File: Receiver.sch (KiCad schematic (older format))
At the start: 29 parts, among them J1 +12V, J2 -12V, J3 GND, J4 OUTPUT, U1 TL074 (ggf. durch TLV4172IPWR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

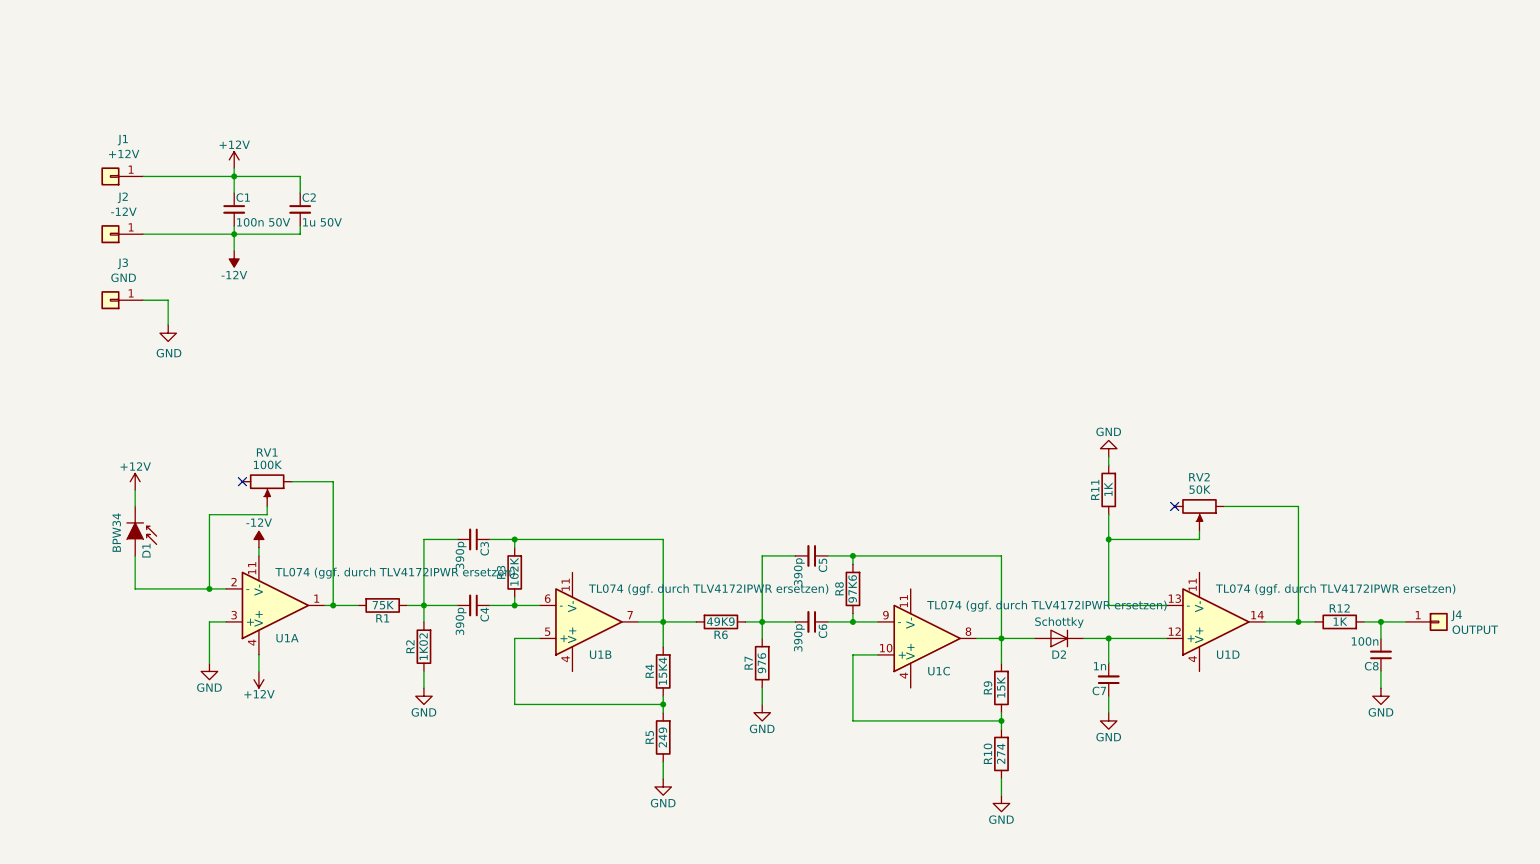
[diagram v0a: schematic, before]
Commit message: Update schematic and pcb
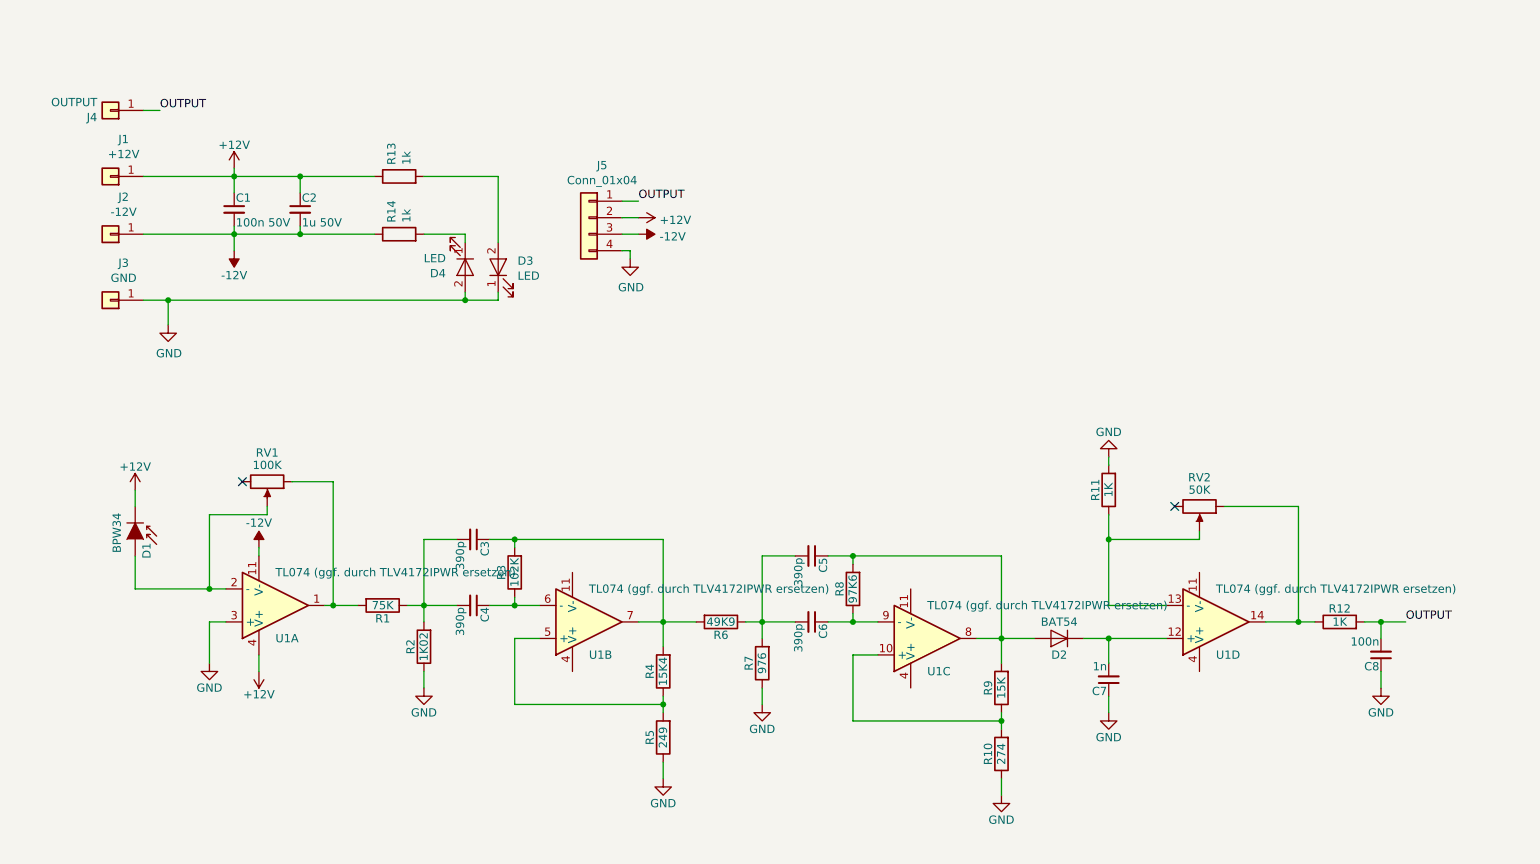
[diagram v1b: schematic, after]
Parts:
- added D3, D4: LED, LEDs:LED_0603, symbol device:LED
- added J5: Conn_01x04, Pin_Headers:Pin_Header_Straight_1x04_Pitch2.54mm, symbol Connector:Conn_01x04
- added R13, R14: 1k, Resistors_SMD:R_0603, symbol device:R
- D2: value Schottky -> BAT54; footprint Diodes_SMD:D_SOD-123 -> Diodes_SMD:D_SOT-23_ANK
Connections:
- net +12V: now also J5.2 (Pin_2), R13.1
- net -12V: now also J5.3 (Pin_3), R14.1
- net GND: now also D3.1 (K), D4.2 (A), J5.4 (Pin_4)
- net OUTPUT: now reaches C8.2, J4.1 (Pin_1), R12.2
- net OUTPUT: now also J5.1 (Pin_1)
- new net: D3.2 (A), R13.2
- new net: D4.1 (K), R14.2
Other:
- moved on the sheet: J4
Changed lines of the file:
@@
 P 7700 4300
 F 0 "D2" H 7700 4400 50  0000 C CNN
-F 1 "Schottky " H 7700 4200 50  0000 C CNN
-F 2 "Diodes_SMD:D_SOD-123" H 7700 4300 50  0001 C CNN
+F 1 "BAT54" H 7700 4200 50  0000 C CNN
+F 2 "Diodes_SMD:D_SOT-23_ANK" H 7700 4300 50  0001 C CNN
 F 3 "" H 7700 4300 50  0001 C CNN
 	1    7700 4300
@@
 L Connector:Conn_01x01 J4
 U 1 1 5B03236E
-P 10000 4200
-F 0 "J4" H 10080 4242 50  0000 L CNN
-F 1 "OUTPUT" H 10080 4151 50  0000 L CNN
-F 2 "optoreceiver:Hirschmann_MST201" H 10000 4200 50  0001 C CNN
-F 3 "~" H 10000 4200 50  0001 C CNN
-	1    10000 4200
-	1    0    0    -1
+P 1950 1100
+F 0 "J4" H 2030 1142 50  0000 L CNN
+F 1 "OUTPUT" H 2030 1051 50  0000 L CNN
+F 2 "optoreceiver:Hirschmann_MST201" H 1950 1100 50  0001 C CNN
+F 3 "~" H 1950 1100 50  0001 C CNN
+	1    1950 1100
+	-1   0    0    1
 $EndComp
 Wire Wire Line
@@
 Wire Wire Line
 	2300 2250 2300 2400
+$Comp
+L device:LED D3
+U 1 1 5B14466C
+P 4300 2050
+F 0 "D3" V 4338 1933 50  0000 R CNN
+F 1 "LED" V 4247 1933 50  0000 R CNN
+F 2 "LEDs:LED_0603" H 4300 2050 50  0001 C CNN
+F 3 "~" H 4300 2050 50  0001 C CNN
+	1    4300 2050
+	0    -1   -1   0
+$EndComp
+Wire Wire Line
+	4300 2200 4300 2250
+$Comp
+L device:R R13
+U 1 1 5B14B3A1
+P 3700 1500
+F 0 "R13" H 3770 1546 50  0000 L CNN
+F 1 "1k" H 3770 1455 50  0000 L CNN
+F 2 "Resistors_SMD:R_0603" V 3630 1500 50  0001 C CNN
+F 3 "" H 3700 1500 50  0001 C CNN
+	1    3700 1500
+	0    -1   -1   0
+$EndComp
+$Comp
+L Connector:Conn_01x04 J5
+U 1 1 5B150E6D
+P 4850 1750
+F 0 "J5" H 4770 2067 50  0000 C CNN
+F 1 "Conn_01x04" H 4770 1976 50  0000 C CNN
+F 2 "Pin_Headers:Pin_Header_Straight_1x04_Pitch2.54mm" H 4850 1750 50  0001 C CNN
+F 3 "~" H 4850 1750 50  0001 C CNN
+	1    4850 1750
+	-1   0    0    -1
+$EndComp
+Text Label 2250 1100 0    50   ~ 0
+OUTPUT
+Wire Wire Line
+	2250 1100 2150 1100
+Text Label 9800 4200 0    50   ~ 0
+OUTPUT
+$Comp
+L power:GND #PWR0101
+U 1 1 5B156865
+P 5100 2000
+F 0 "#PWR0101" H 5100 1750 50  0001 C CNN
+F 1 "GND" H 5105 1827 50  0000 C CNN
+F 2 "" H 5100 2000 50  0001 C CNN
+F 3 "" H 5100 2000 50  0001 C CNN
+	1    5100 2000
+	1    0    0    -1
+$EndComp
+Wire Wire Line
+	5050 1950 5100 1950
+Wire Wire Line
+	5100 1950 5100 2000
+$Comp
+L power:+12V #PWR0102
+U 1 1 5B15914A
+P 5150 1750
+F 0 "#PWR0102" H 5150 1600 50  0001 C CNN
+F 1 "+12V" V 5165 1878 50  0000 L CNN
+F 2 "" H 5150 1750 50  0001 C CNN
+F 3 "" H 5150 1750 50  0001 C CNN
+	1    5150 1750
+	0    1    1    0
+$EndComp
+$Comp
+L power:-12V #PWR15
+U 1 1 5B15948E
+P 5150 1850
+F 0 "#PWR15" H 5150 1950 50  0001 C CNN
+F 1 "-12V" V 5165 1978 50  0000 L CNN
+F 2 "" H 5150 1850 50  0001 C CNN
+F 3 "" H 5150 1850 50  0001 C CNN
+	1    5150 1850
+	0    1    1    0
+$EndComp
+Wire Wire Line
+	5150 1850 5050 1850
+Wire Wire Line
+	5150 1750 5050 1750
+Text Label 5150 1650 0    50   ~ 0
+OUTPUT
+Wire Wire Line
+	5150 1650 5050 1650
+Wire Wire Line
+	3100 1500 3550 1500
+Connection ~ 3100 1500
+Wire Wire Line
+	2300 2250 4100 2250
+Connection ~ 2300 2250
+$Comp
+L device:R R14
+U 1 1 5B17749B
+P 3700 1850
+F 0 "R14" H 3770 1896 50  0000 L CNN
+F 1 "1k" H 3770 1805 50  0000 L CNN
+F 2 "Resistors_SMD:R_0603" V 3630 1850 50  0001 C CNN
+F 3 "" H 3700 1850 50  0001 C CNN
+	1    3700 1850
+	0    -1   -1   0
+$EndComp
+Wire Wire Line
+	3550 1850 3100 1850
+Connection ~ 3100 1850
+$Comp
+L device:LED D4
+U 1 1 5B182712
+P 4100 2050
+F 0 "D4" V 4138 1933 50  0000 R CNN
+F 1 "LED" V 4047 1933 50  0000 R CNN
+F 2 "LEDs:LED_0603" H 4100 2050 50  0001 C CNN
+F 3 "~" H 4100 2050 50  0001 C CNN
+	1    4100 2050
+	0    1    1    0
+$EndComp
+Wire Wire Line
+	4100 2200 4100 2250
+Connection ~ 4100 2250
+Wire Wire Line
+	4100 2250 4300 2250
+Wire Wire Line
+	3850 1850 4100 1850
+Wire Wire Line
+	4100 1850 4100 1900
+Wire Wire Line
+	3850 1500 4300 1500
+Wire Wire Line
+	4300 1500 4300 1900
 $EndSCHEMATC

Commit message: Add files via upload
- Platzierung und Silkscreen angepasst
- 3D Modelle ergänzt
- aktuelle Renderbilder erzeugt
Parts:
- C1, C2, C3, C4, C5, C6, C7, C8: symbol device:C_Small -> Device:C_Small
- D2: symbol device:D -> Device:D
- D3, D4: symbol device:LED -> Device:LED
- J1, J2, J3, J4: symbol Connector:Conn_01x01 -> Connector:Conn_01x01_Female
- J5: symbol Connector:Conn_01x04 -> Connector:Conn_01x04_Female
- R1, R10, R11, R12, R13, R14, R2, R3, R4, R5, R6, R7, R8, R9: symbol device:R -> Device:R
- RV1, RV2: footprint SparkFun-Electromechanical:TRIM_POT -> User-Submitted:BOURNS-3362P_pot
- U1: footprint Package_SO:TSSOP-14_4.4x5mm_P0.65mm -> Package_SO:SOIC-14_3.9x8.7mm_P1.27mm
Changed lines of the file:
@@
 F 0 "U1" H 2950 4300 50  0000 L CNN
 F 1 "TL074 (ggf. durch TLV4172IPWR ersetzen)" H 2950 3900 50  0000 L CNN
-F 2 "Package_SO:TSSOP-14_4.4x5mm_P0.65mm" H 2900 4200 50  0001 C CNN
+F 2 "Package_SO:SOIC-14_3.9x8.7mm_P1.27mm" H 2900 4200 50  0001 C CNN
 F 3 "" H 3000 4300 50  0001 C CNN
 	1    2950 4100
@@
 $EndComp
 $Comp
-L power:-12V #PWR5
+L power:-12V #PWR05
 U 1 1 5AEAF2F4
 P 2850 3750
-F 0 "#PWR5" H 2850 3850 50  0001 C CNN
+F 0 "#PWR05" H 2850 3850 50  0001 C CNN
 F 1 "-12V" H 2850 3900 50  0000 C CNN
 F 2 "" H 2850 3750 50  0001 C CNN
@@
 	1    0    0    -1
 $EndComp
-Wire Wire Line
-	2850 4400 2850 4500
-Wire Wire Line
-	2850 3750 2850 3800
 Wire Wire Line
 	2550 4000 2650 4000
@@
 F 0 "U1" H 4850 4400 50  0000 L CNN
 F 1 "TL074 (ggf. durch TLV4172IPWR ersetzen)" H 4850 4000 50  0000 L CNN
-F 2 "Package_SO:TSSOP-14_4.4x5mm_P0.65mm" H 4800 4300 50  0001 C CNN
+F 2 "Package_SO:SOIC-14_3.9x8.7mm_P1.27mm" H 4800 4300 50  0001 C CNN
 F 3 "" H 4900 4400 50  0001 C CNN
 	2    4850 4200
@@
 $EndComp
 $Comp
-L device:R R1
+L Device:R R1
 U 1 1 5AEAF541
 P 3600 4100
@@
 $EndComp
 $Comp
-L device:R R2
+L Device:R R2
 U 1 1 5AEAF581
 P 3850 4350
@@
 	3850 3700 3850 4100
 $Comp
-L device:C_Small C4
+L Device:C_Small C4
 U 1 1 5AEAF686
 P 4150 4100
@@
 $EndComp
 $Comp
-L device:C_Small C3
+L Device:C_Small C3
 U 1 1 5AEAF715
 P 4150 3700
@@
 	4250 4100 4400 4100
 $Comp
-L device:R R3
+L Device:R R3
 U 1 1 5AEAF96B
 P 4400 3900
@@
 Connection ~ 4400 3700
 $Comp
-L device:R R4
+L Device:R R4
 U 1 1 5AEAFA8E
 P 5300 4500
@@
 $EndComp
 $Comp
-L device:R R5
+L Device:R R5
 U 1 1 5AEAFAD7
 P 5300 4900
@@
 F 0 "U1" H 6900 4500 50  0000 L CNN
 F 1 "TL074 (ggf. durch TLV4172IPWR ersetzen)" H 6900 4100 50  0000 L CNN
-F 2 "Package_SO:TSSOP-14_4.4x5mm_P0.65mm" H 6850 4400 50  0001 C CNN
+F 2 "Package_SO:SOIC-14_3.9x8.7mm_P1.27mm" H 6850 4400 50  0001 C CNN
 F 3 "" H 6950 4500 50  0001 C CNN
 	3    6900 4300
@@
 $EndComp
 $Comp
-L device:R R6
+L Device:R R6
 U 1 1 5AEAFDA7
 P 5650 4200
@@
 $EndComp
 $Comp
-L device:R R7
+L Device:R R7
 U 1 1 5AEAFDAD
 P 5900 4450
@@
 	5900 3800 5900 4200
 $Comp
-L device:C_Small C6
+L Device:C_Small C6
 U 1 1 5AEAFDBC
 P 6200 4200
@@
 $EndComp
 $Comp
-L device:C_Small C5
+L Device:C_Small C5
 U 1 1 5AEAFDC2
 P 6200 3800
@@
 	6300 4200 6450 4200
 $Comp
-L device:R R8
+L Device:R R8
 U 1 1 5AEAFDC9
 P 6450 4000
@@
 Connection ~ 6450 3800
 $Comp
-L device:R R9
+L Device:R R9
 U 1 1 5AEAFDD8
 P 7350 4600
@@
 $EndComp
 $Comp
-L device:R R10
+L Device:R R10
 U 1 1 5AEAFDDE
 P 7350 5000
@@
 	7350 5150 7350 5250
 $Comp
-L device:C_Small C1
+L Device:C_Small C1
 U 1 1 5AEAFE56
 P 2700 1700
@@
 	2700 1450 2700 1500
 $Comp
-L power:-12V #PWR2
+L power:-12V #PWR02
 U 1 1 5AEAFF86
 P 2700 1950
-F 0 "#PWR2" H 2700 2050 50  0001 C CNN
+F 0 "#PWR02" H 2700 2050 50  0001 C CNN
 F 1 "-12V" H 2700 2100 50  0000 C CNN
 F 2 "" H 2700 1950 50  0001 C CNN
@@
 F 0 "RV2" V 8375 3500 50  0000 C CNN
 F 1 "50K" V 8450 3500 50  0000 C CNN
-F 2 "SparkFun-Electromechanical:TRIM_POT" H 8550 3500 50  0001 C CNN
+F 2 "User-Submitted:BOURNS-3362P_pot" H 8550 3500 50  0001 C CNN
 F 3 "" H 8550 3500 50  0001 C CNN
 	1    8550 3500
@@
 $EndComp
 $Comp
-L device:D D2
+L Device:D D2
 U 1 1 5AEB05C3
 P 7700 4300
@@
 $EndComp
 $Comp
-L device:C_Small C7
+L Device:C_Small C7
 U 1 1 5AEB0668
 P 8000 4550
@@
 Wire Wire Line
 	7850 4300 8000 4300
-$Comp
-L Receiver-rescue:TL074-linear U1
-U 4 1 5AEB085F
-P 8650 4200
-F 0 "U1" H 8650 4400 50  0000 L CNN
-F 1 "TL074 (ggf. durch TLV4172IPWR ersetzen)" H 8650 4000 50  0000 L CNN
-F 2 "Package_SO:TSSOP-14_4.4x5mm_P0.65mm" H 8600 4300 50  0001 C CNN
-F 3 "" H 8700 4400 50  0001 C CNN
-	4    8650 4200
-	1    0    0    1
-$EndComp
 Connection ~ 8000 4300
 Wire Wire Line
@@
 	8950 4200 9150 4200
 $Comp
-L device:R R12
+L Device:R R12
 U 1 1 5AEB0CD1
 P 9400 4200
@@
 Connection ~ 9150 4200
 $Comp
-L device:C_Small C8
+L Device:C_Small C8
 U 1 1 5AEB0DB0
 P 9650 4400
@@
 F 0 "RV1" V 2725 3350 50  0000 C CNN
 F 1 "100K" V 2800 3350 50  0000 C CNN
-F 2 "SparkFun-Electromechanical:TRIM_POT" H 2900 3350 50  0001 C CNN
+F 2 "User-Submitted:BOURNS-3362P_pot" H 2900 3350 50  0001 C CNN
 F 3 "" H 2900 3350 50  0001 C CNN
 	1    2900 3350
@@
 	2100 4000 2550 4000
 $Comp
-L device:R R11
+L Device:R R11
 U 1 1 5AF96B45
 P 8000 3400
@@
 NoConn ~ 8400 3500
 $Comp
-L device:C_Small C2
+L Device:C_Small C2
 U 1 1 5AFB3597
 P 3100 1700
@@
 $EndComp
 $Comp
-L Connector:Conn_01x01 J1
+L Connector:Conn_01x01_Female J1
 U 1 1 5B031E2F
 P 1950 1500
@@
 $EndComp
 $Comp
-L Connector:Conn_01x01 J3
+L Connector:Conn_01x01_Female J3
 U 1 1 5B0321C2
 P 1950 2250
@@
 $EndComp
 $Comp
-L Connector:Conn_01x01 J2
+L Connector:Conn_01x01_Female J2
 U 1 1 5B032258
 P 1950 1850
@@
 $EndComp
 $Comp
-L Connector:Conn_01x01 J4
+L Connector:Conn_01x01_Female J4
 U 1 1 5B03236E
 P 1950 1100
@@
 	2300 2250 2300 2400
 $Comp
-L device:LED D3
+L Device:LED D3
 U 1 1 5B14466C
 P 4300 2050
@@
 	4300 2200 4300 2250
 $Comp
-L device:R R13
+L Device:R R13
 U 1 1 5B14B3A1
 P 3700 1500
@@
 $EndComp
 $Comp
-L Connector:Conn_01x04 J5
+L Connector:Conn_01x04_Female J5
 U 1 1 5B150E6D
 P 4850 1750
@@
 $EndComp
 $Comp
-L power:-12V #PWR15
+L power:-12V #PWR015
 U 1 1 5B15948E
 P 5150 1850
-F 0 "#PWR15" H 5150 1950 50  0001 C CNN
+F 0 "#PWR015" H 5150 1950 50  0001 C CNN
 F 1 "-12V" V 5165 1978 50  0000 L CNN
 F 2 "" H 5150 1850 50  0001 C CNN
@@
 Connection ~ 2300 2250
 $Comp
-L device:R R14
+L Device:R R14
 U 1 1 5B17749B
 P 3700 1850
@@
 Connection ~ 3100 1850
 $Comp
-L device:LED D4
+L Device:LED D4
 U 1 1 5B182712
 P 4100 2050
@@
 Wire Wire Line
 	4300 1500 4300 1900
+Wire Wire Line
+	2850 4400 2850 4500
+Wire Wire Line
+	2850 3750 2850 3800
+$Comp
+L power:+12V #PWR0104
+U 1 1 5B16DE44
+P 4750 4500
+F 0 "#PWR0104" H 4750 4350 50  0001 C CNN
+F 1 "+12V" H 4750 4640 50  0000 C CNN
+F 2 "" H 4750 4500 50  0001 C CNN
+F 3 "" H 4750 4500 50  0001 C CNN
+	1    4750 4500
+	-1   0    0    1
+$EndComp
+$Comp
+L Receiver-rescue:TL074-linear U1
+U 4 1 5AEB085F
+P 8650 4200
+F 0 "U1" H 8650 4400 50  0000 L CNN
+F 1 "TL074 (ggf. durch TLV4172IPWR ersetzen)" H 8650 4000 50  0000 L CNN
+F 2 "Package_SO:SOIC-14_3.9x8.7mm_P1.27mm" H 8600 4300 50  0001 C CNN
+F 3 "" H 8700 4400 50  0001 C CNN
+	4    8650 4200
+	1    0    0    1
+$EndComp
 $EndSCHEMATC
